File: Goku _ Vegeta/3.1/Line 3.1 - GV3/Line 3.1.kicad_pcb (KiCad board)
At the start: 2 copper layers, 112 parts, among them J1 Solenoid, J10 RIGHT HEADERS, J11 Kicker Voltmeter, J3 Motor 1, J4 Motor 3, J5 Motor 2, J6 Motor 4, J7 BATTERY POWER, J8 I2C TO MASTER, J9 LEFT HEADERS, Q2 BSC040N10NS5, U1 LM2587S-ADJ, U10 TPS62132, U11 TPS62133, U2 TB67H420FTG Dual/Single Motor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, U3 TB67H420FTG Dual/Single Motor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, U4 TB67H420FTG Dual/Single Motor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, U5 TB67H420FTG Dual/Single Motor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, U7 NXV55UNR, U9 DEV-16771

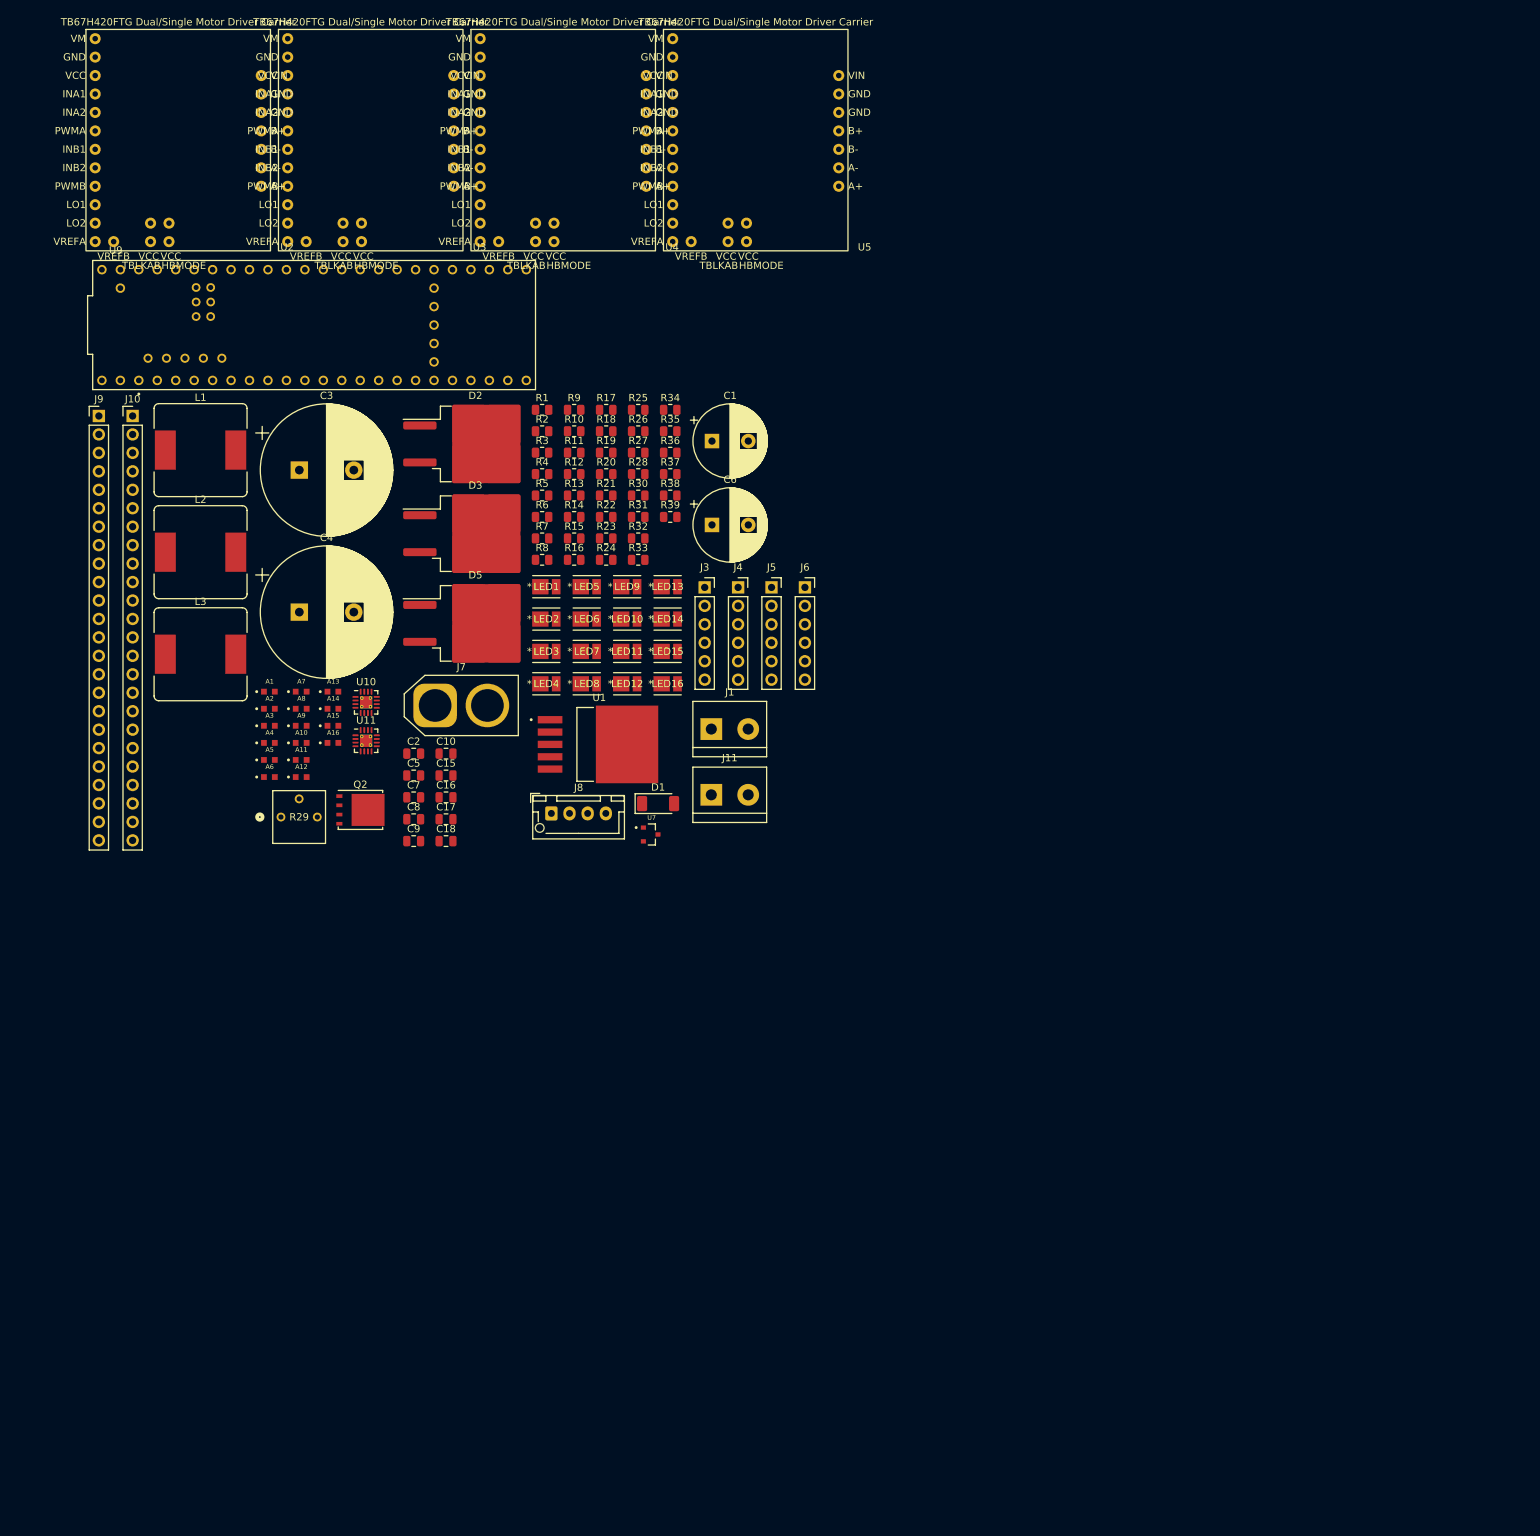
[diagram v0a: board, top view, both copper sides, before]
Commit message: move to 3.1
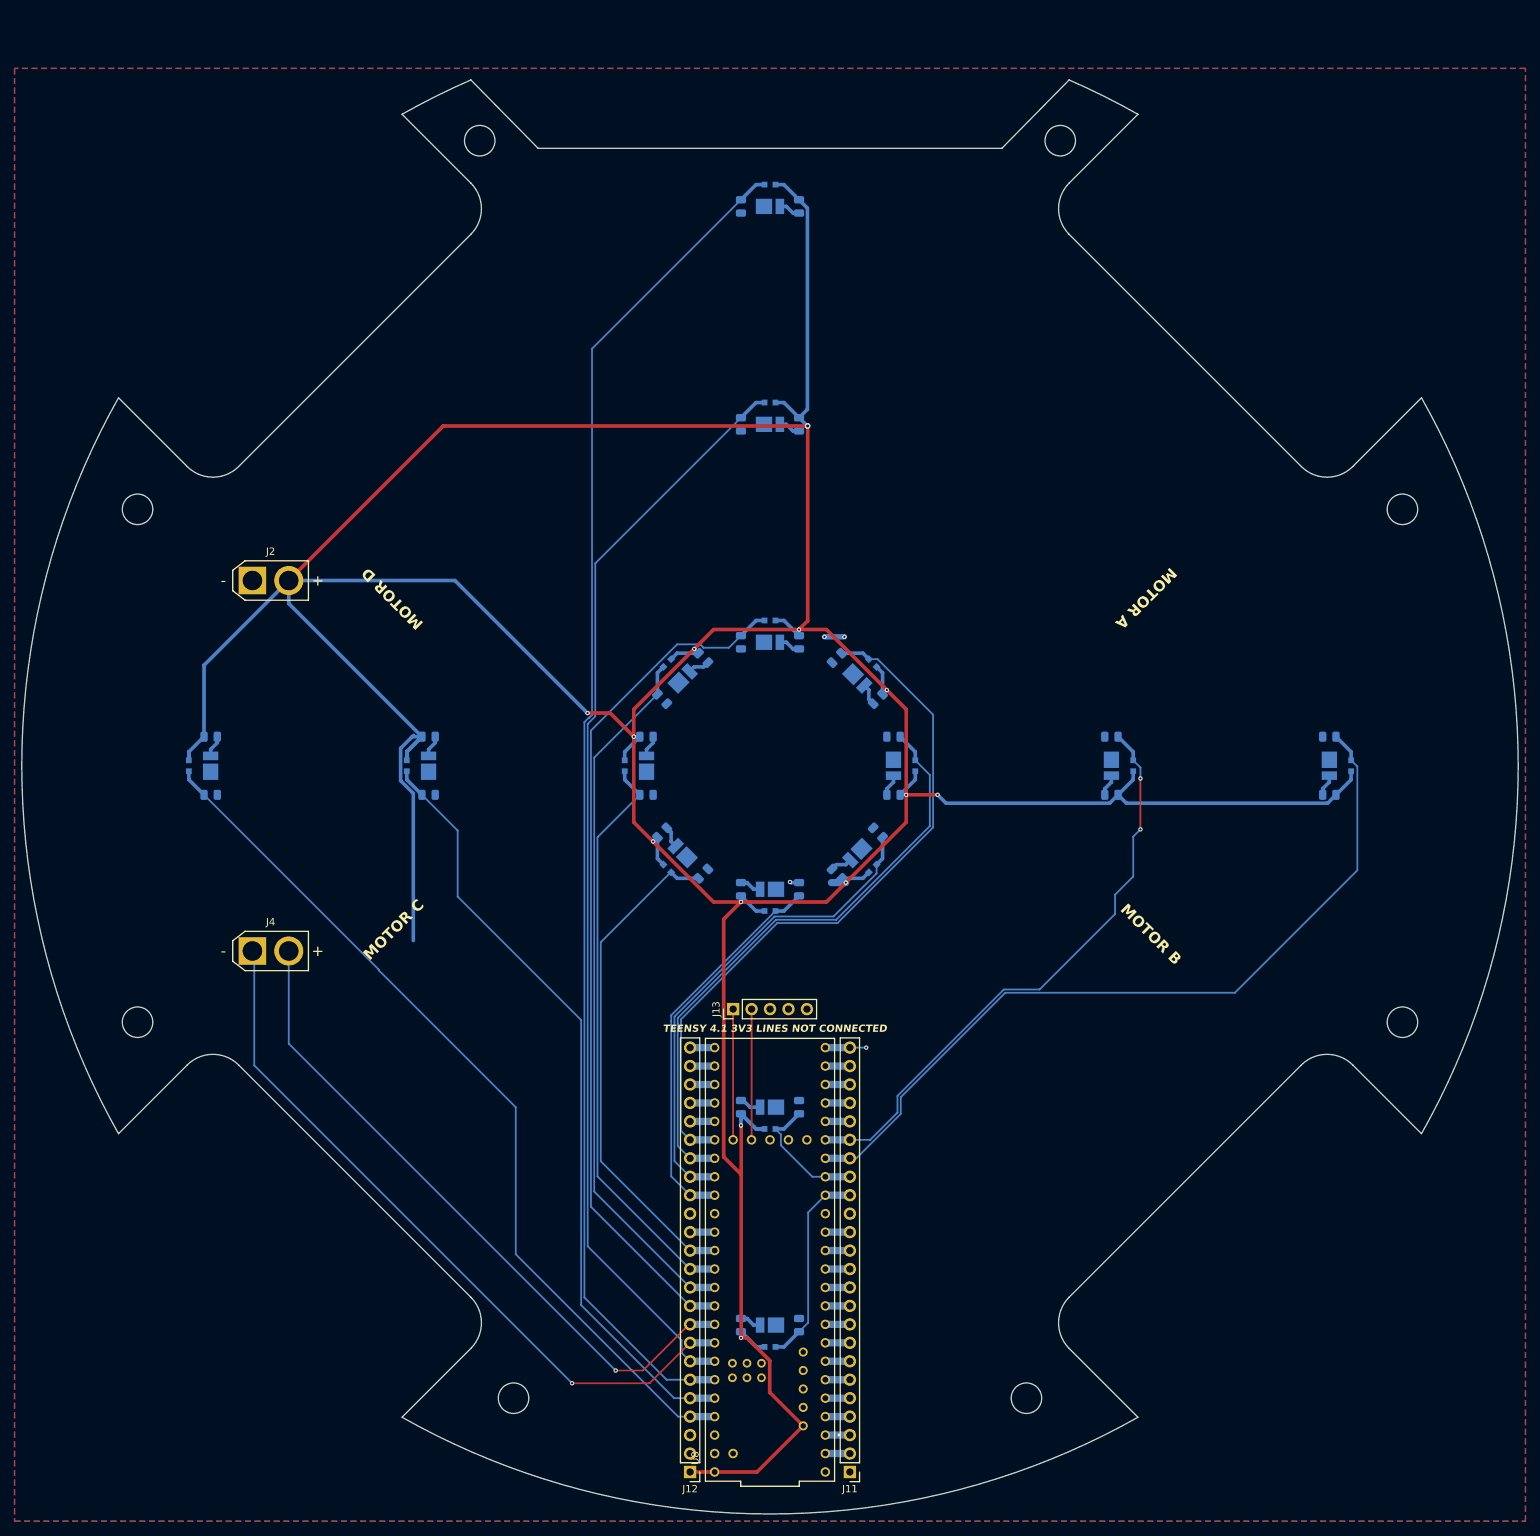
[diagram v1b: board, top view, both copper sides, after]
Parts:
- removed C1, C6: 100uF, Capacitor_THT:CP_Radial_D10.0mm_P5.00mm
- removed C10, C16: 0.1uF, Capacitor_SMD:C_0805_2012Metric
- removed C15, C8: 10uF, Capacitor_SMD:C_0805_2012Metric
- removed C17, C9: 3.3nF, Capacitor_SMD:C_0805_2012Metric
- removed C18, C7: 22uF, Capacitor_SMD:C_0805_2012Metric
- removed C2, C5: 1uF, Capacitor_SMD:C_0805_2012Metric
- removed C3, C4: 560uF, Capacitor_THT:CP_Radial_D18.0mm_P7.50mm
- removed D1: SS510, Diode_SMD:D_SOD-128
- removed D2, D3, D5: STTH2002G-TR, Package_TO_SOT_SMD:TO-263-2
- removed J1: Solenoid, TerminalBlock:TerminalBlock_bornier-2_P5.08mm
- removed J10: RIGHT HEADERS, Connector_PinHeader_2.54mm:PinHeader_1x24_P2.54mm_Vertical
- removed J3: Motor 1, Connector_PinSocket_2.54mm:PinSocket_1x06_P2.54mm_Vertical
- removed J5: Motor 2, Connector_PinSocket_2.54mm:PinSocket_1x06_P2.54mm_Vertical
- removed J6: Motor 4, Connector_PinSocket_2.54mm:PinSocket_1x06_P2.54mm_Vertical
- removed J7: BATTERY POWER, Connector_AMASS:AMASS_XT60-F_1x02_P7.20mm_Vertical
- removed J8: I2C TO MASTER, Connector_JST:JST_XH_B4B-XH-AM_1x04_P2.50mm_Vertical
- removed J9: LEFT HEADERS, Connector_PinHeader_2.54mm:PinHeader_1x24_P2.54mm_Vertical
- removed L1: 56uH, Inductor_SMD:L_Bourns_SRR1260
- removed L2, L3: 2.2uH, Inductor_SMD:L_Bourns_SRR1260
- removed Q2: BSC040N10NS5, Package_TO_SOT_SMD:TDSON-8-1
- removed R33, R35, R37, R39: 10K, Resistor_SMD:R_0805_2012Metric
- removed R34, R36, R38: 12R, Resistor_SMD:R_0805_2012Metric
- removed U1: LM2587S-ADJ, LM2587S-ADJ:VREG_TPS79625KTTR
- removed U10: TPS62132, Package_DFN_QFN:VQFN-16-1EP_3x3mm_P0.5mm_EP1.68x1.68mm_ThermalVias
- removed U11: TPS62133, Package_DFN_QFN:VQFN-16-1EP_3x3mm_P0.5mm_EP1.68x1.68mm_ThermalVias
- removed U2, U3, U4, U5: TB67H420FTG Dual/Single Motor Driver Carrier, TB67H420FTG Dual_Single Motor Driver Carrier:TB67H420FTG DualSingle Motor Driver Carrier
- removed U7: NXV55UNR, NXV55UNR:TRANS_BC846B,215
- removed U9: DEV-16771, DEV-16771:MODULE_DEV-16771
- added J12: RIGHT HEADERS, Connector_PinHeader_2.54mm:PinHeader_1x24_P2.54mm_Vertical, F.Cu at (139.0, 247.2)
- added J13: MID HEADERS, Connector_PinHeader_2.54mm:PinHeader_1x05_P2.54mm_Vertical, F.Cu at (144.9, 183.5)
- added J2: BACKUP 5V, Connector_AMASS:AMASS_XT30U-F_1x02_P5.0mm_Vertical, F.Cu at (78.8, 124.5)
- added U8: DEV-16771, DEV-16771:MODULE_DEV-16771, F.Cu at (150.0, 218.0)
- A1, A10, A11, A12, A13, A14, A15, A16, A2, A3, A4, A5, A6, A7, A8, A9, LED1, LED10, LED11, LED12, LED13, LED14, LED15, LED16, LED2, LED3, LED4, LED5, LED6, LED7, LED8, LED9, R10, R12, R14, R16, R26, R28: moved to B.Cu
- J11: value Kicker Voltmeter -> LEFT HEADERS; footprint TerminalBlock:TerminalBlock_bornier-2_P5.08mm -> Connector_PinHeader_2.54mm:PinHeader_1x24_P2.54mm_Vertical
- J4: value Motor 3 -> I2C; footprint Connector_PinSocket_2.54mm:PinSocket_1x06_P2.54mm_Vertical -> Connector_AMASS:AMASS_XT30U-F_1x02_P5.0mm_Vertical
- R1: value 2K94 -> 36R; moved to B.Cu
- R11, R13, R15, R25, R27, R31, R9: value 12R -> 10K; moved to B.Cu
- R17, R19, R21, R23, R4, R6: value 12R -> 36R; moved to B.Cu
- R18, R20, R22, R24, R5, R7, R8: value 10K -> 36R; moved to B.Cu
- R2: value 57K -> 36R; moved to B.Cu
- R29: value CT6EP103 -> 10K; footprint POT_CT-6EP_NDC:POT_CT-6EP_NDC -> Resistor_SMD:R_0805_2012Metric; moved to B.Cu
- R3: value 1K5 -> 36R; moved to B.Cu
- R30, R32: value 100K -> 10K; moved to B.Cu
- moved A2 149.1 mm to (230.0, 150.0), turned to 90 degrees
- moved R11 124.0 mm to (154.0, 227.0), turned to -90 degrees
- moved R3 123.2 mm to (146.0, 227.0), turned to 90 degrees
- moved R2 119.4 mm to (227.0, 154.0), turned to 180 degrees
- moved A6 118.9 mm to (200.0, 150.0), turned to 90 degrees
- moved R10 112.1 mm to (227.0, 146.0)
- moved A3 109.8 mm to (150.0, 230.0)
- moved LED2 109.7 mm to (227.0, 150.0), turned to -90 degrees
- moved A1 98.1 mm to (150.0, 70.0), turned to 180 degrees
- moved LED3 97.7 mm to (150.0, 227.0), turned to 180 degrees
- moved J11 95.2 mm to (161.0, 247.2), turned to 180 degrees
- moved A7 88.3 mm to (150.0, 200.0)
- moved R6 87.2 mm to (197.0, 154.0), turned to 180 degrees
- moved A5 84.7 mm to (150.0, 100.0), turned to 180 degrees
- moved A11 84.5 mm to (170.0, 150.0), turned to 90 degrees
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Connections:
- A1 pad 1: +3V3 -> +5V
- A1 pad 2: /SEN1 -> /21
- A10 pad 1: +3V3 -> +5V
- A10 pad 2: /SEN1 -> /38
- A11 pad 1: +3V3 -> +5V
- A11 pad 2: /SEN1 -> /39
- A12 pad 1: +3V3 -> +5V
- A12 pad 2: /SEN1 -> /40
- A13 pad 1: +3V3 -> +5V
- A13 pad 2: /SEN1 -> /41
- A14 pad 1: +3V3 -> +5V
- A14 pad 2: /SEN1 -> /14
- A15 pad 1: +3V3 -> +5V
- A15 pad 2: /SEN1 -> /15
- A16 pad 1: +3V3 -> +5V
- A16 pad 2: /SEN1 -> /16
- A2 pad 1: +3V3 -> +5V
- A2 pad 2: /SEN1 -> /26
- A3 pad 1: +3V3 -> +5V
- A3 pad 2: /SEN1 -> /24
- A4 pad 1: +3V3 -> +5V
- A4 pad 2: /SEN1 -> /23
- A5 pad 1: +3V3 -> +5V
- A5 pad 2: /SEN1 -> /20
- A6 pad 1: +3V3 -> +5V
- A6 pad 2: /SEN1 -> /27
- A7 pad 1: +3V3 -> +5V
- A7 pad 2: /SEN1 -> /25
- A8 pad 1: +3V3 -> +5V
- A8 pad 2: /SEN1 -> /22
- A9 pad 1: +3V3 -> +5V
- A9 pad 2: /SEN1 -> /17
- J11 pad 1: Net-(D1-K) -> GND
- J11 pad 2: GND -> /0
- J4 pad 1: Net-(J4-Pin_1) -> /19
- J4 pad 2: Net-(J4-Pin_2) -> /18
- LED1 pad 1: /MSFTDRN -> GND
- LED10 pad 1: /MSFTDRN -> GND
- LED11 pad 1: /MSFTDRN -> GND
- LED12 pad 1: /MSFTDRN -> GND
- LED13 pad 1: /MSFTDRN -> GND
- LED14 pad 1: /MSFTDRN -> GND
- LED15 pad 1: /MSFTDRN -> GND
- LED16 pad 1: /MSFTDRN -> GND
- LED2 pad 1: /MSFTDRN -> GND
- LED3 pad 1: /MSFTDRN -> GND
- LED4 pad 1: /MSFTDRN -> GND
- LED5 pad 1: /MSFTDRN -> GND
- LED6 pad 1: /MSFTDRN -> GND
- LED7 pad 1: /MSFTDRN -> GND
- LED8 pad 1: /MSFTDRN -> GND
- LED9 pad 1: /MSFTDRN -> GND
- R1 pad 1: Net-(U1-COMP) -> +5V
- R1 pad 2: Net-(C2-Pad1) -> Net-(LED1-Pad2)
- R10 pad 2: /SEN1 -> /26
- R11 pad 1: +3V3 -> GND
- R11 pad 2: Net-(LED4-Pad2) -> /24
- R12 pad 2: /SEN1 -> /23
- R13 pad 1: +3V3 -> GND
- R13 pad 2: Net-(LED5-Pad2) -> /20
- R14 pad 2: /SEN1 -> /27
- R15 pad 1: +3V3 -> GND
- R15 pad 2: Net-(LED6-Pad2) -> /25
- R16 pad 2: /SEN1 -> /22
- R17 pad 1: +3V3 -> +5V
- R17 pad 2: Net-(LED7-Pad2) -> Net-(LED9-Pad2)
- R18 pad 1: GND -> +5V
- R18 pad 2: /SEN1 -> Net-(LED10-Pad2)
- R19 pad 1: +3V3 -> +5V
- R19 pad 2: Net-(LED8-Pad2) -> Net-(LED11-Pad2)
- R2 pad 1: Net-(D1-K) -> +5V
- R2 pad 2: Net-(R2-Pad2) -> Net-(LED2-Pad2)
- R20 pad 1: GND -> +5V
- R20 pad 2: /SEN1 -> Net-(LED12-Pad2)
- R21 pad 1: +3V3 -> +5V
- R21 pad 2: Net-(LED9-Pad2) -> Net-(LED13-Pad2)
- R22 pad 1: GND -> +5V
- R22 pad 2: /SEN1 -> Net-(LED14-Pad2)
- R23 pad 1: +3V3 -> +5V
- R23 pad 2: Net-(LED10-Pad2) -> Net-(LED15-Pad2)
- R24 pad 1: GND -> +5V
- R24 pad 2: /SEN1 -> Net-(LED16-Pad2)
- R25 pad 1: +3V3 -> GND
- R25 pad 2: Net-(LED11-Pad2) -> /17
- R26 pad 2: /SEN1 -> /38
- R27 pad 1: +3V3 -> GND
- R27 pad 2: Net-(LED12-Pad2) -> /39
- R28 pad 2: /SEN1 -> /40
- R29 pad 1: Net-(U1-FB) -> GND
- R29 pad 2: Net-(U1-FB) -> /41
- R3 pad 1: Net-(U1-FB) -> +5V
- R3 pad 2: GND -> Net-(LED3-Pad2)
- R30 pad 1: Net-(U10-PG) -> GND
- R30 pad 2: +3V3 -> /14
- R31 pad 1: +3V3 -> GND
- R31 pad 2: Net-(LED13-Pad2) -> /15
- R32 pad 1: Net-(U11-PG) -> GND
- R32 pad 2: +5V -> /16
- R4 pad 1: +3V3 -> +5V
- R4 pad 2: Net-(LED1-Pad2) -> Net-(LED4-Pad2)
- R5 pad 1: GND -> +5V
- R5 pad 2: /SEN1 -> Net-(LED5-Pad2)
- R6 pad 1: +3V3 -> +5V
- R6 pad 2: Net-(LED2-Pad2) -> Net-(LED6-Pad2)
- R7 pad 1: GND -> +5V
- R7 pad 2: /2 -> Net-(LED7-Pad2)
- R8 pad 1: GND -> +5V
- R8 pad 2: /SEN1 -> Net-(LED8-Pad2)
- R9 pad 1: +3V3 -> GND
- R9 pad 2: Net-(LED3-Pad2) -> /21
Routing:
- net +5V: track 0.00 -> 664.1 mm, vias 0 -> 13
- net /21: track 0.00 -> 186.8 mm
- net /20: track 0.00 -> 152.0 mm
- net /23: track 0.00 -> 121.8 mm
- net /17: track 0.00 -> 118.8 mm
- net /26: track 0.00 -> 110.6 mm
- net /22: track 0.00 -> 107.1 mm
- net /19: track 0.00 -> 99.7 mm, vias 0 -> 1
- net /16: track 0.00 -> 98.2 mm
- net /38: track 0.00 -> 97.8 mm
- net /18: track 0.00 -> 92.8 mm, vias 0 -> 1
- net /39: track 0.00 -> 83.0 mm
- net /27: track 0.00 -> 81.2 mm, vias 0 -> 2
- net /15: track 0.00 -> 80.5 mm
- net /14: track 0.00 -> 68.7 mm
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- added copper zone on B.Cu, net GND
- added copper zone on F.Cu, net GND
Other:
- board outline added: 206 x 197.4 mm
- board text added: "Designed by Hugh Phan - September 2023"
- board text added: "Fort Street's Team Silverback Hugh Phan Jayden Nguyen Issey Lee Jack Sumner KZ KC"
- board text added: "MOTOR A"
- board text added: "MOTOR B"
- board text added: "MOTOR C"
- board text added: "MOTOR D"
- board text added: "TEENSY 4.1 3V3 LINES NOT CONNECTED"
